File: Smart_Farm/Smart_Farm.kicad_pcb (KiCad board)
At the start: 2 copper layers, 125.5 x 108 mm, 23 parts, among them J1 EJ508A, J2 Screw_Terminal_01x03, Q1 2N3904, U1 ESP32-DEVKITC-32D, U2 LCD 16x2 I2C, U3 SOIL SENSOR, U4 RTC, U5 Relay Module

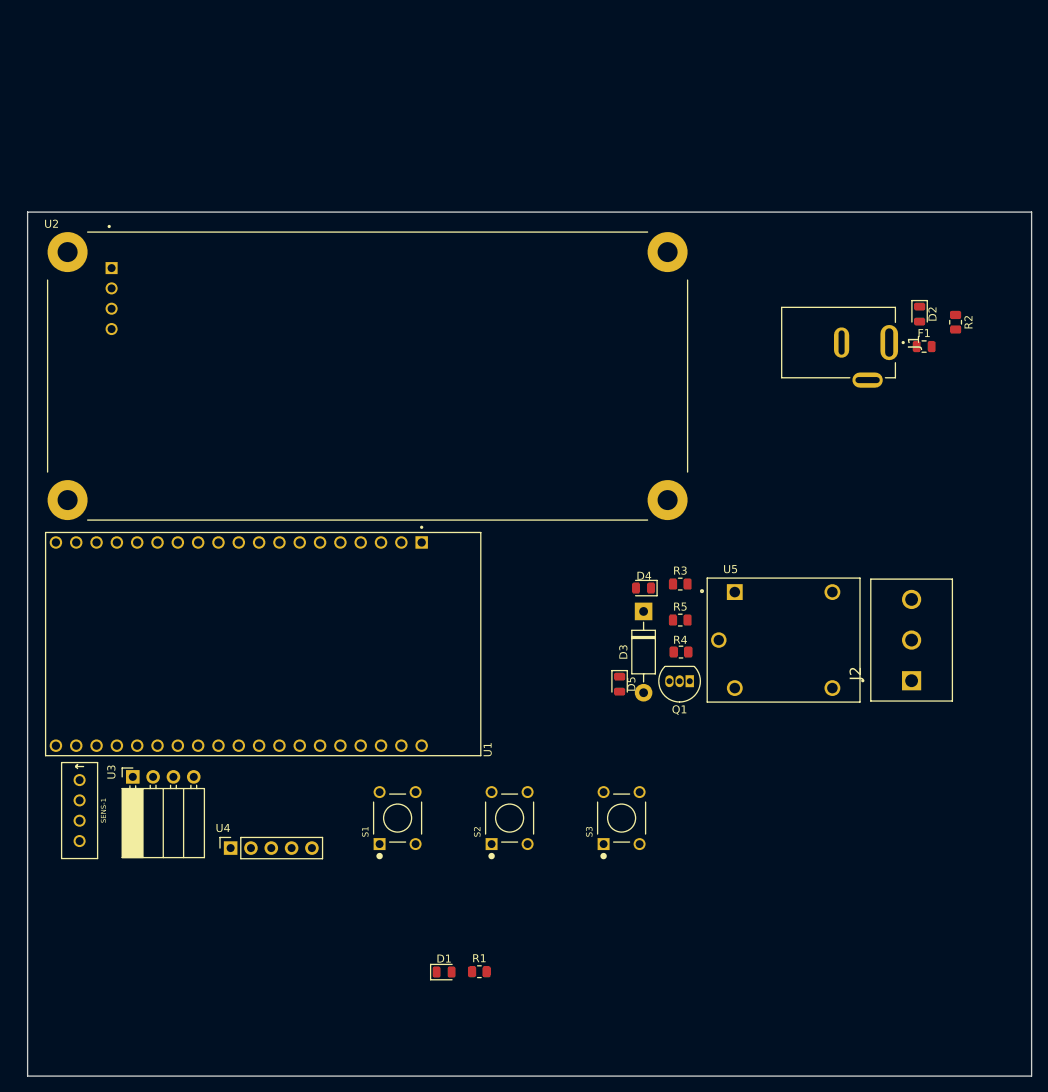
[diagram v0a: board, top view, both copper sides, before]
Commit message: Update Schematic and PCB
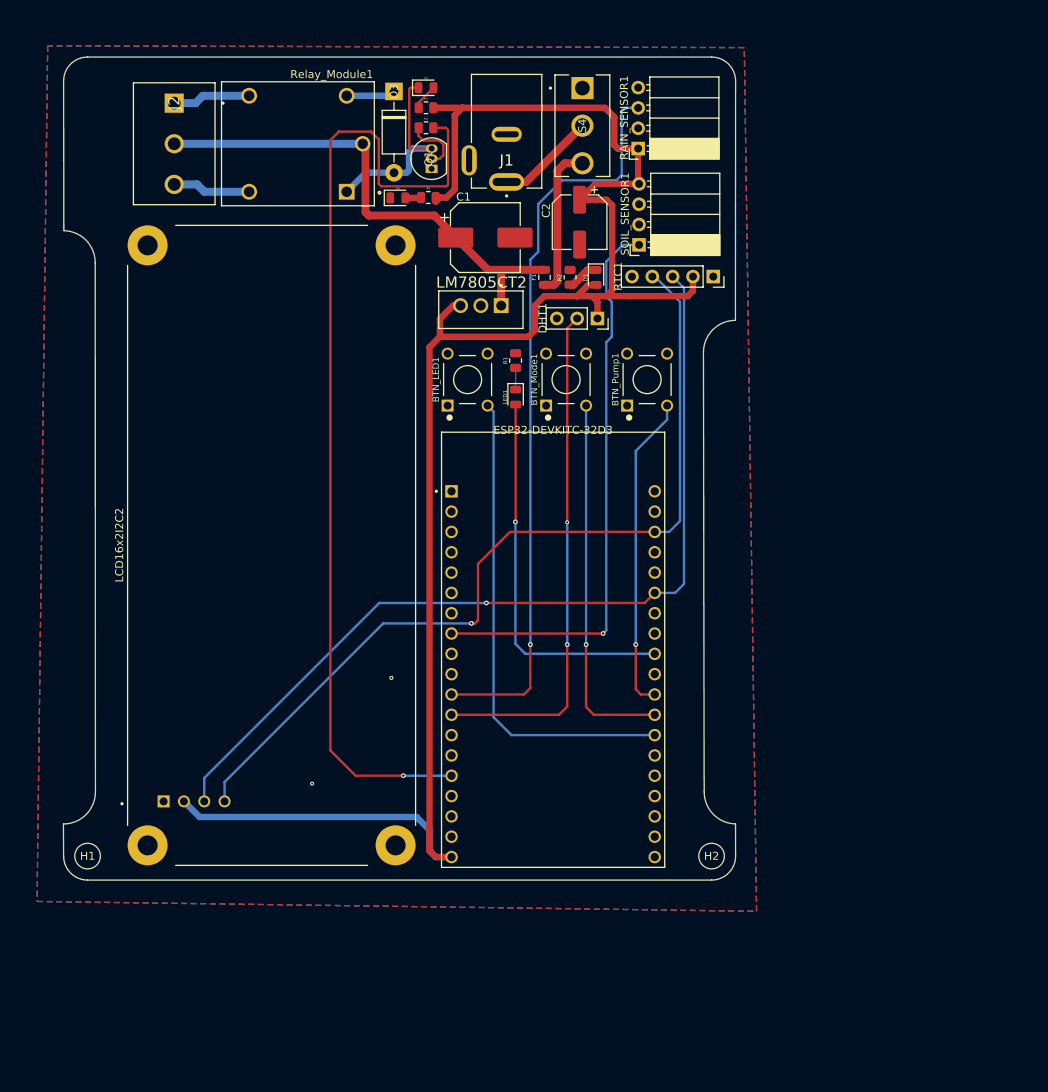
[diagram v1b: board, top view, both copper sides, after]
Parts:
- removed SENS-1: DHT11, Smart_Farm:SENSOR-DHT11
- added C1: C_Polarized_Small_US, Capacitor_SMD:CP_Elec_8x10.5, F.Cu at (152.7, 59.7)
- added C2: C_Polarized_Small_US, Capacitor_SMD:CP_Elec_6.3x5.4, F.Cu at (164.5, 57.8)
- added DHT1: DHT11, Connector_PinSocket_2.54mm:PinSocket_1x03_P2.54mm_Vertical, F.Cu at (166.7, 69.8)
- added H1: MountingHole, MountingHole:MountingHole_3.2mm_M3_ISO14580, F.Cu at (103.0, 137.0)
- added H2: MountingHole, MountingHole:MountingHole_3.2mm_M3_ISO14580, F.Cu at (181.0, 137.0)
- added LM7805CT2: LM7805CT, Smart_Farm:LM7805CT, F.Cu at (152.2, 68.2)
- added RAIN_SENSOR1: RAIN SENSOR, Connector_PinSocket_2.54mm:PinSocket_1x04_P2.54mm_Horizontal, F.Cu at (171.8, 48.6)
- added S4: 100SP1T1B4M2QE, Smart_Farm:SW_100SP1T1B4M2QE, F.Cu at (164.8, 45.7)
- R1, R2, R3, R4, R5: value 1k -> R
- moved J2 117.1 mm to (113.8, 42.9), turned to -90 degrees
- moved RTC1 93.5 mm to (181.2, 64.6), turned to -90 degrees
- moved SOIL_SENSOR1 91.8 mm to (171.9, 60.6), turned to 180 degrees
- moved Relay_Module1 86.8 mm to (129.3, 48.0), turned to 180 degrees
- moved D5 78.4 mm to (145.3, 41.0), turned to 0 degrees
- moved R1 76.5 mm to (156.5, 75.1), turned to -90 degrees
- moved R4 72.9 mm to (145.3, 46.0), turned to 180 degrees
- moved LED1 72.4 mm to (156.5, 79.6), turned to -90 degrees
- moved D3 72.1 mm to (141.3, 41.4)
- moved Q1 71.7 mm to (146.0, 51.1), turned to 90 degrees
- moved R3 67.5 mm to (145.3, 43.5)
- moved R5 61.5 mm to (145.6, 54.7)
- moved D4 57.6 mm to (141.8, 54.7), turned to 0 degrees
- moved BTN_Pump1 57.4 mm to (172.9, 77.4)
- moved BTN_LED1 55.5 mm to (150.5, 77.4)
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- renumbered S1 to BTN_LED1, S3 to BTN_Mode1, S2 to BTN_Pump1, D2 to D1, U1 to ESP32-DEVKITC-32D3, U2 to LCD16x2I2C2, D1 to LED1, U4 to RTC1, U5 to Relay_Module1, U3 to SOIL_SENSOR1
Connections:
- BTN_LED1 pad 2: /IO_33 -> /IO_04
- ESP32-DEVKITC-32D3 pad J2-10: /IO_26 -> unconnected-(ESP32-DEVKITC-32D3-IO26-PadJ2-10)
- ESP32-DEVKITC-32D3 pad J2-11: unconnected-(U1-IO27-PadJ2-11) -> /IO_27
- ESP32-DEVKITC-32D3 pad J2-15: unconnected-(U1-IO13-PadJ2-15) -> /IO_13
- ESP32-DEVKITC-32D3 pad J2-5: /IO_34 -> unconnected-(ESP32-DEVKITC-32D3-IO34-PadJ2-5)
- ESP32-DEVKITC-32D3 pad J3-9: unconnected-(U1-IO18-PadJ3-9) -> /IO_18
- F1 pad 1: +5V -> +12V
- J1 pad 1: Net-(F1-Pad2) -> Net-(J1-Pad1)
- J2 pad 2: Net-(J2-Pin_2) -> +12V
- LED1 pad 2: /IO_04 -> /IO_18
- R4 pad 1: /IO_26 -> /IO_13
- Relay_Module1 pad COM: Net-(J2-Pin_2) -> +12V
- SOIL_SENSOR1 pad 1: /IO_34 -> /IO_33
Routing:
- net +5V: track 0.00 -> 227.0 mm
- net /IO_13: track 0.00 -> 122.9 mm, vias 0 -> 1
- net /IO_21: track 0.00 -> 112.0 mm, vias 0 -> 1
- net /IO_22: track 0.00 -> 109.2 mm, vias 0 -> 1
- net /IO_27: track 0.00 -> 93.4 mm, vias 0 -> 1
- net /IO_33: track 0.00 -> 71.1 mm, vias 0 -> 1
- net /IO_14: track 0.00 -> 63.8 mm, vias 0 -> 2
- net +12V: track 0.00 -> 62.3 mm
- net /IO_04: track 0.00 -> 60.3 mm
- net /IO_18: track 0.00 -> 47.8 mm, vias 0 -> 1
- net /IO_16: track 0.00 -> 46.9 mm, vias 0 -> 1
- net /IO_17: track 0.00 -> 39.7 mm, vias 0 -> 1
- net Net-(D3-A): track 0.00 -> 25.5 mm
- net Net-(F1-Pad2): track 0.00 -> 19.4 mm
- net Net-(J1-Pad1): track 0.00 -> 12.4 mm
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- added copper zone on B.Cu, net GND
- added copper zone on F.Cu, net GND
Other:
- board size 125.5 x 108 mm -> 84 x 102.9 mm
- board text added: "SmartFarm PCB"

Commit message: Update files
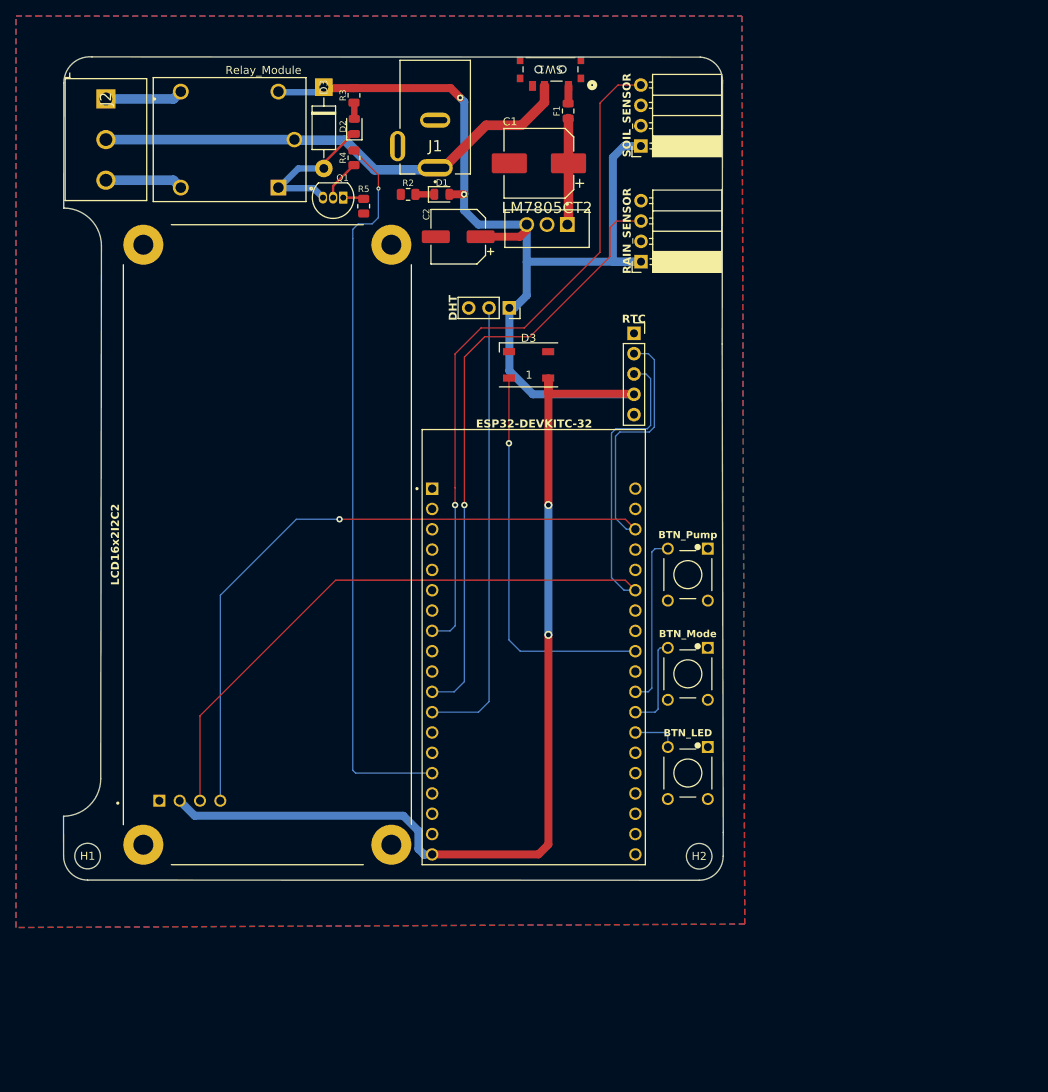
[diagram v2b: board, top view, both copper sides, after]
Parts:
- removed D4, LED1: LED, LED_SMD:LED_0805_2012Metric
- removed R1: R, Resistor_SMD:R_0805_2012Metric
- removed S4: 100SP1T1B4M2QE, Smart_Farm:SW_100SP1T1B4M2QE
- added D3: WS2812B, LED_SMD:LED_WS2812B_PLCC4_5.0x5.0mm_P3.2mm, F.Cu at (158.1, 75.6)
- added SW1: MK-12C02-G020, Smart_Farm:MK-12C02-G020_GSW, F.Cu at (160.9, 38.7)
- C1: value C_Polarized_Small_US -> 470uF
- C2: value C_Polarized_Small_US -> 100uF
- R2, R3, R4: value R -> 1k
- R5: value R -> 10k
- moved BTN_LED 56.4 mm to (178.0, 126.6), turned to -90 degrees
- moved BTN_Mode 39.8 mm to (178.0, 114.2), turned to -90 degrees
- moved BTN_Pump 24.9 mm to (178.0, 101.8), turned to -90 degrees
- moved R2 22.7 mm to (143.1, 54.3), turned to 0 degrees
- moved D1 21.9 mm to (147.3, 54.3), turned to 0 degrees
- moved F1 21.0 mm to (163.1, 43.9), turned to 90 degrees
- moved C2 15.3 mm to (149.3, 59.6), turned to 180 degrees
- moved RAIN_SENSOR 14.1 mm to (172.2, 62.7)
- moved LM7805CT2 13.1 mm to (160.4, 58.1)
- moved SOIL_SENSOR 12.4 mm to (172.2, 48.2)
- moved RTC 12.2 mm to (171.3, 71.7), turned to 0 degrees
- moved Q1 11.6 mm to (135.0, 54.7), turned to 180 degrees
- moved C1 11.4 mm to (159.4, 50.4), turned to 180 degrees
- moved DHT 11.1 mm to (155.7, 68.5)
- moved D2 10.2 mm to (136.3, 45.8), turned to 90 degrees
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- renumbered BTN_LED1 to BTN_LED, BTN_Mode1 to BTN_Mode, BTN_Pump1 to BTN_Pump, D5 to D2, DHT1 to DHT, ESP32-DEVKITC-32D3 to ESP32-DEVKITC-32, RAIN_SENSOR1 to RAIN_SENSOR, RTC1 to RTC, Relay_Module1 to Relay_Module, SOIL_SENSOR1 to SOIL_SENSOR
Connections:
- D3 pad 1: Net-(D3-K) -> +5V
- J1 pad 1: Net-(J1-Pad1) -> /+12V Power
- J1 pad 3: GND -> unconnected-(J1-Pad3)
- J2 pad 1: Net-(J2-Pin_1) -> GND
- J2 pad 2: +12V -> /+12V Power
- Q1 pad 1: GND -> Net-(Q1-E)
- R5 pad 1: Net-(D4-A) -> GND
- R5 pad 2: +5V -> Net-(Q1-E)
- RAIN_SENSOR pad 2: unconnected-(RAIN_SENSOR1-AO-Pad2) -> GND
- RAIN_SENSOR pad 4: GND -> unconnected-(RAIN_SENSOR1-AO-Pad4)
- RTC pad 1: GND -> unconnected-(RTC1-DS-Pad1)
- RTC pad 2: +5V -> /IO_22
- RTC pad 4: /IO_22 -> +5V
- RTC pad 5: unconnected-(RTC1-DS-Pad5) -> GND
- Relay_Module pad A2: Net-(D3-K) -> +5V
- Relay_Module pad COM: +12V -> /+12V Power
- Relay_Module pad NO: Net-(J2-Pin_1) -> GND
- SOIL_SENSOR pad 1: /IO_33 -> +5V
- SOIL_SENSOR pad 2: unconnected-(SOIL_SENSOR1-DO-Pad2) -> GND
- SOIL_SENSOR pad 3: GND -> unconnected-(SOIL_SENSOR1-DO-Pad3)
- SOIL_SENSOR pad 4: +5V -> /IO_33
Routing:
- net /+12V Power: track 0.00 -> 63.1 mm
- net /IO_04: track 60.3 -> 5.66 mm
- net +12V: track 62.3 -> 13.3 mm
- net /IO_16: track 46.9 -> 11.7 mm, vias 1 -> 0
- net /IO_13: track 122.9 -> 91.6 mm
- net +5V: track 227.0 -> 247.8 mm, vias 0 -> 4
- net /IO_17: track 39.7 -> 21.4 mm, vias 1 -> 0
- net Net-(F1-Pad2): track 19.4 -> 2.21 mm
- net /IO_27: track 93.4 -> 76.4 mm
- net /IO_33: track 71.1 -> 85.1 mm
- net Net-(J1-Pad1): track 12.4 -> 0.00 mm
- net Net-(J2-Pin_1): track 9.74 -> 0.00 mm
- net GND: track 0.41 -> 9.74 mm, vias 2 -> 0
- net /IO_14: track 63.8 -> 56.9 mm, vias 2 -> 0
- net Net-(D3-K): track 6.35 -> 0.00 mm
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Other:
- board size 84 x 102.9 mm -> 82.5 x 102.9 mm
